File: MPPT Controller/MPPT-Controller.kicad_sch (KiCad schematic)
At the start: 60 parts, among them J1 Conn_01x02_Pin, J2 Conn_01x02_Pin, J3 Conn_01x02_Pin, J4 Conn_01x02_Pin, J6 Conn_01x02_Pin, J7 Conn_01x02_Pin, J8 Conn_01x02_Pin, M1 Fan_4pin, Q1 IRL540N, SW1 SW_SPDT, U1 ADS1115IDGS, U4 LM1117DT-3.3, U5 LM2596S-ADJ, U6 TC4422, U7 ADS1115IDGS

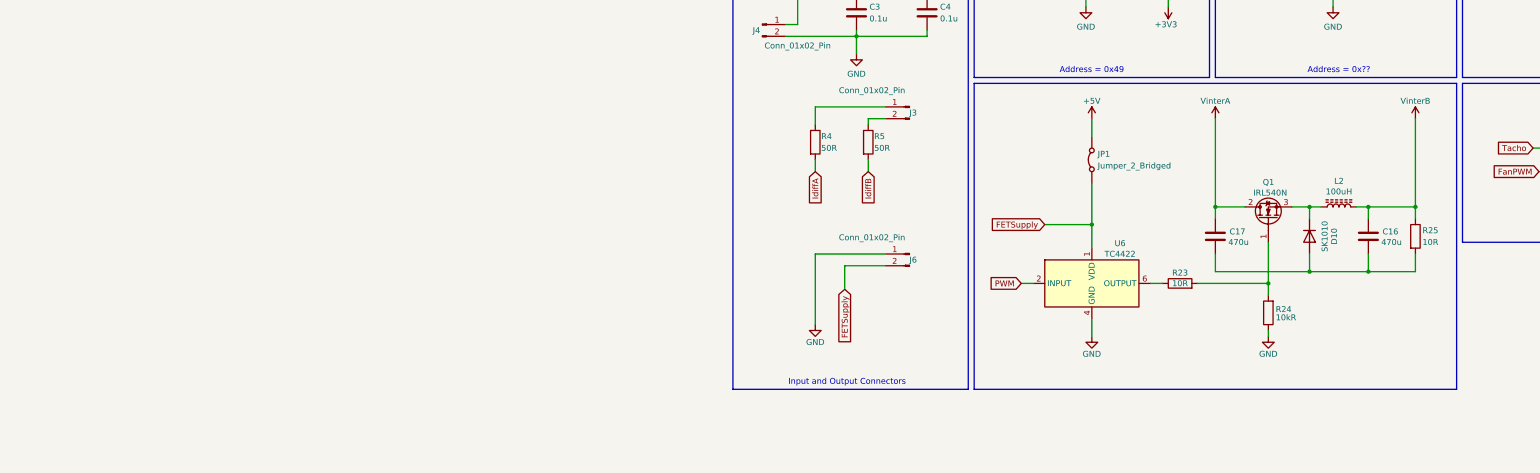
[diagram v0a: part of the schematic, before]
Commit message: Rework
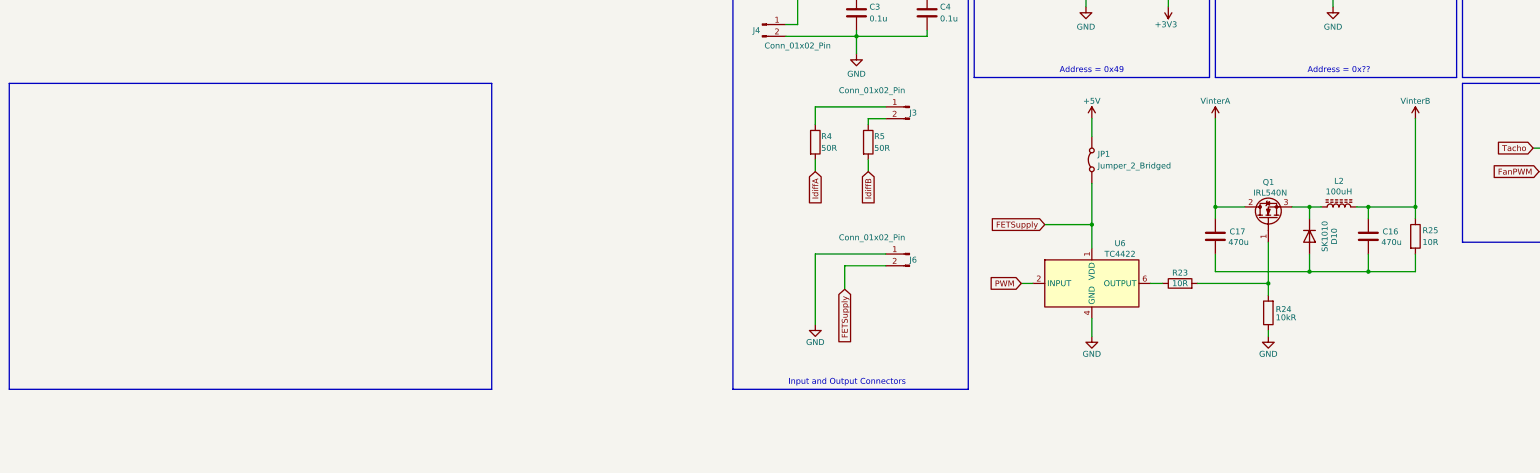
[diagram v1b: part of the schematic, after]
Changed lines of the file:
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@@
 	)
 	(rectangle
-		(start 66.04 130.81)
-		(end 170.18 196.85)
+		(start -38.1 130.81)
+		(end -142.24 196.85)
 		(stroke
 			(width 0)

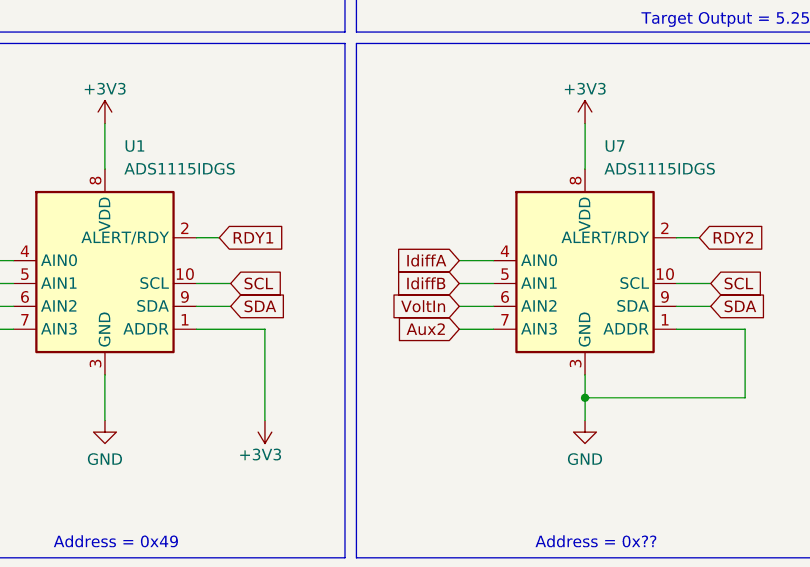
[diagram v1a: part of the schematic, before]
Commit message: Fix Label Name
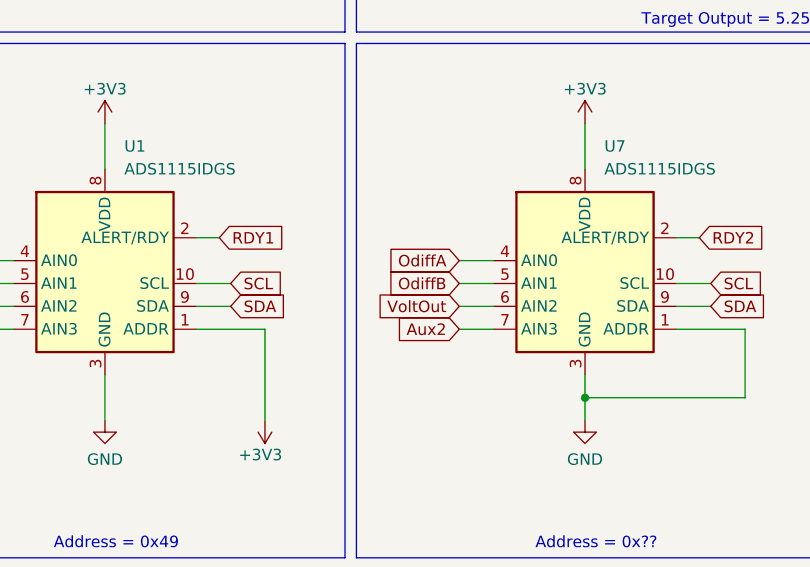
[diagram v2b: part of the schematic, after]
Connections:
- net IdiffA: no longer U7.4 (AIN0)
- net IdiffB: no longer U7.5 (AIN1)
- net OdiffA: now also U7.4 (AIN0)
- net OdiffB: now also U7.5 (AIN1)
- net VoltIn: no longer U7.6 (AIN2)
- new net VoltOut: U7.6 (AIN2)
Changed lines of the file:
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@@
 		)
 	)
-	(global_label "VoltIn"
+	(global_label "VoltOut"
 		(shape input)
 		(at 129.54 101.6 180)
@@
 		)
 		(property "Intersheetrefs" "${INTERSHEET_REFS}"
-			(at 121.1725 101.6 0)
+			(at 119.7211 101.6 0)
 			(effects
 				(font
@@
 		)
 	)
-	(global_label "IdiffA"
+	(global_label "OdiffA"
 		(shape input)
 		(at 129.54 96.52 180)
@@
 		)
 		(property "Intersheetrefs" "${INTERSHEET_REFS}"
-			(at 121.6562 96.52 0)
+			(at 120.9305 96.52 0)
 			(effects
 				(font
@@
 		)
 	)
-	(global_label "IdiffB"
+	(global_label "OdiffB"
 		(shape input)
 		(at 129.54 99.06 180)
@@
 		)
 		(property "Intersheetrefs" "${INTERSHEET_REFS}"
-			(at 121.4748 99.06 0)
-			(effects
-				(font
+			(at 120.7491 99.06 0)
+			(effects
+				(font
